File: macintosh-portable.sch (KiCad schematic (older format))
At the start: 0 parts

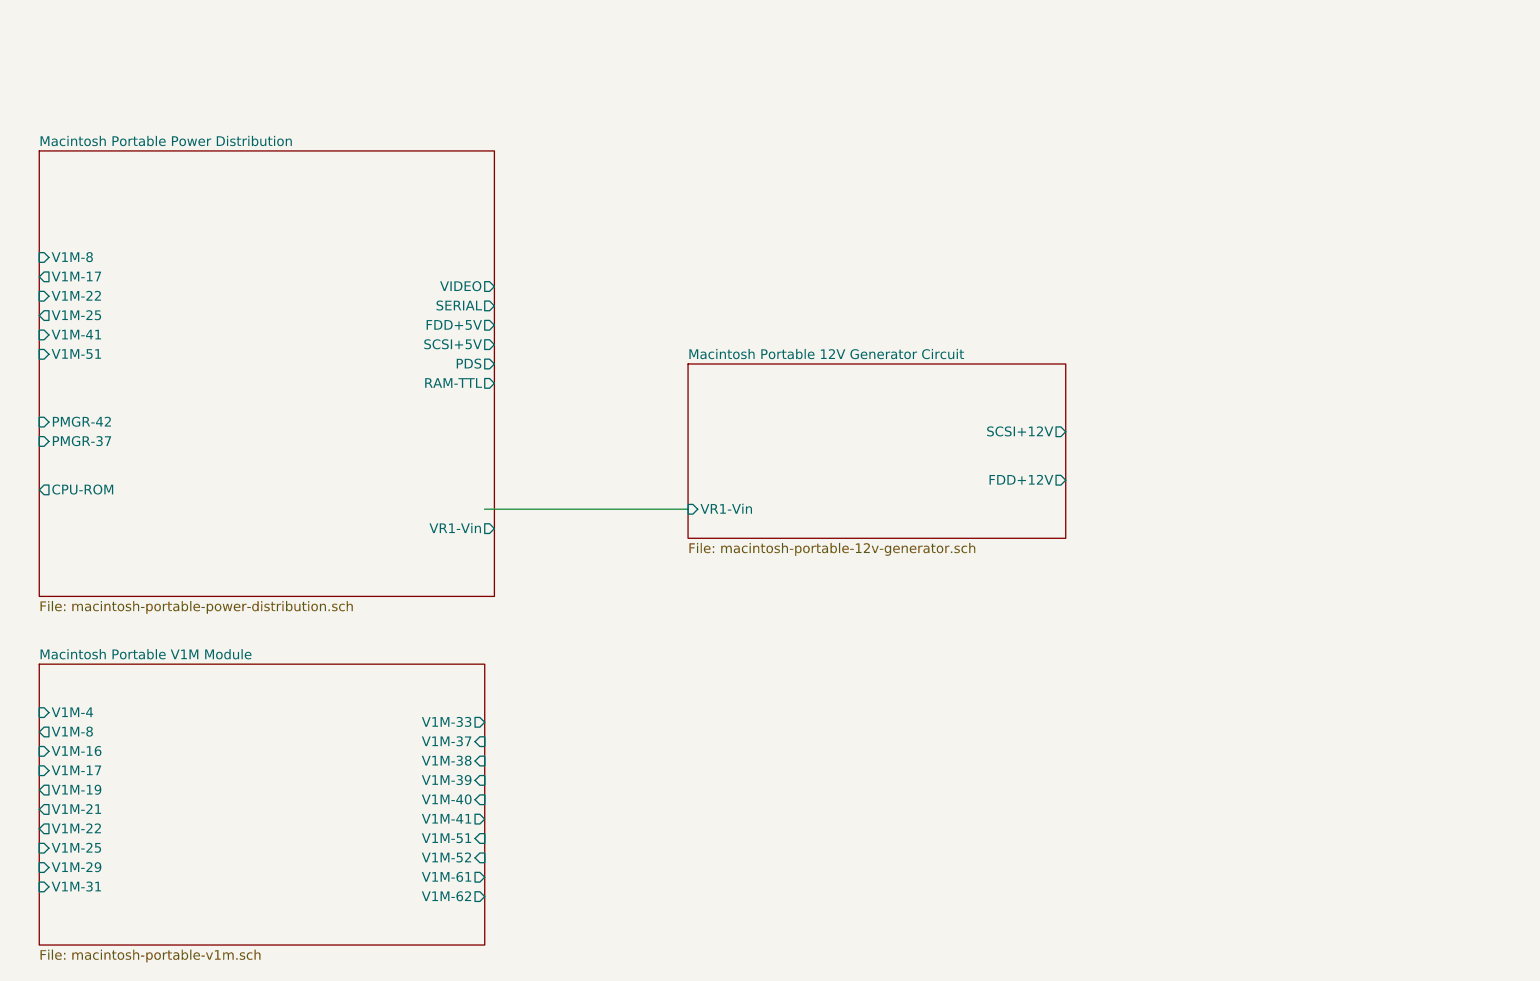
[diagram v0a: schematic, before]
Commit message: Finished V1M, more references on other sheets.
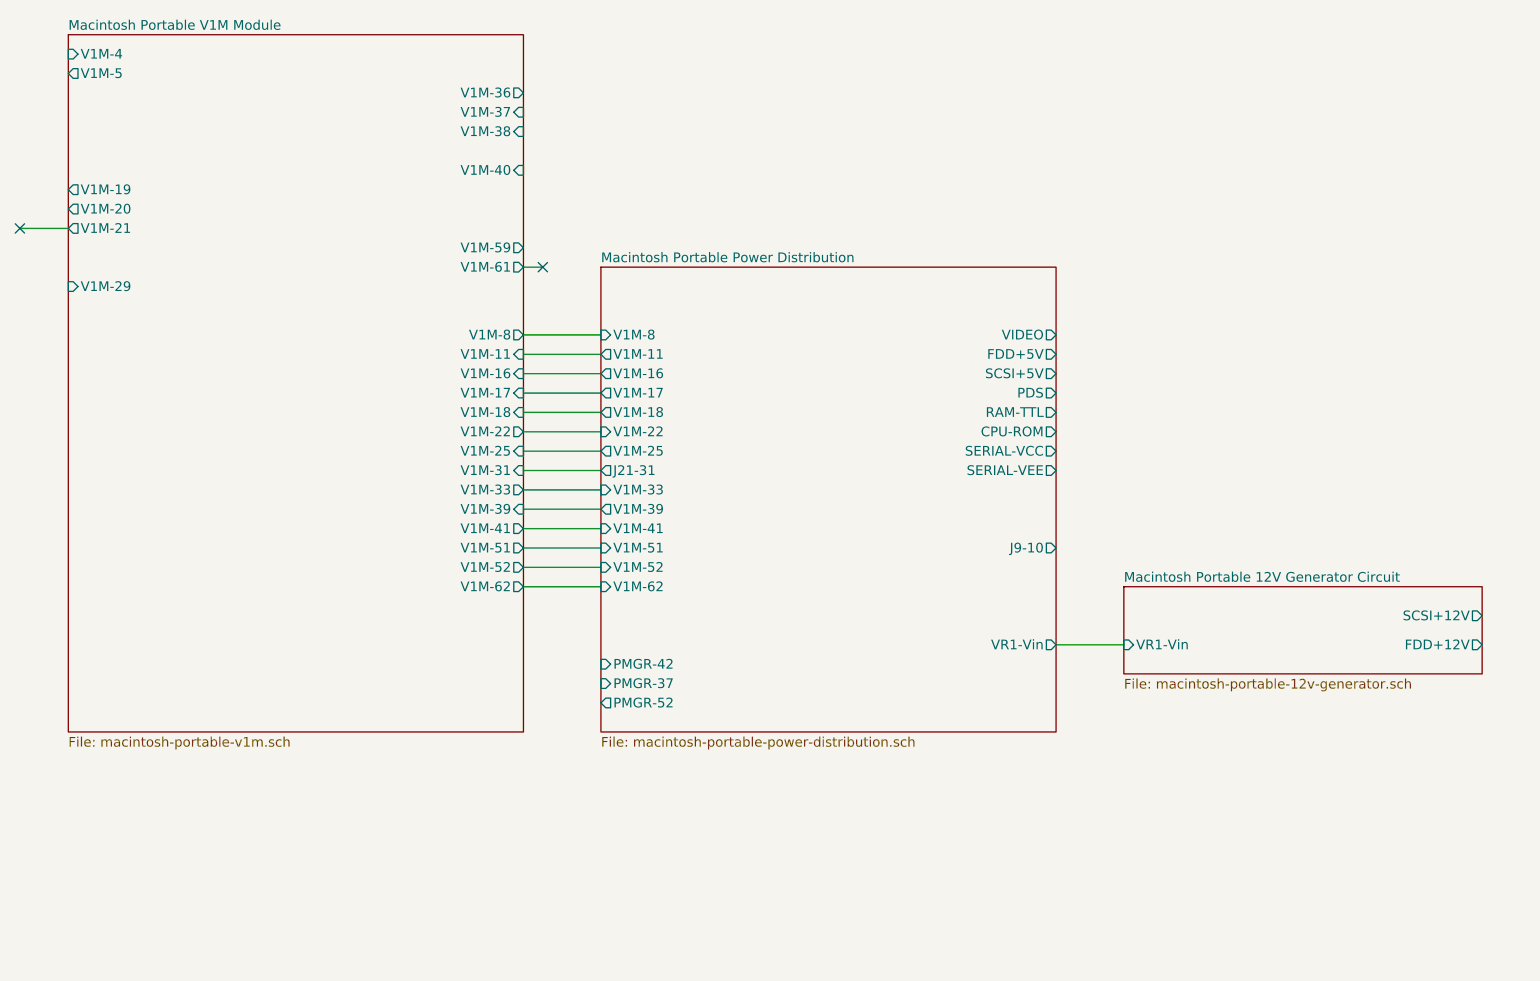
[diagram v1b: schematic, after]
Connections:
- wire segments 1 -> 17
- no-connect marks 0 -> 2
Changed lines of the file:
@@
 encoding utf-8
 Sheet 1 4
-Title ""
-Date ""
-Rev "0.1"
-Comp ""
-Comment1 ""
+Title "Macintosh Portable Power"
+Date "2019-05-27"
+Rev "0.12"
+Comp "https://oldcrap.org"
+Comment1 "Author: Pawel Pieczul"
 Comment2 ""
 Comment3 ""
@@
 $EndDescr
 $Sheet
-S 1200 1500 2350 2300
+S 4100 2100 2350 2400
 U 5CE45908
 F0 "Macintosh Portable Power Distribution" 50
 F1 "macintosh-portable-power-distribution.sch" 50
-F2 "VR1-Vin" O R 3550 3450 50
-F3 "V1M-41" I L 1200 2450 50
-F4 "V1M-51" I L 1200 2550 50
-F5 "PMGR-42" I L 1200 2900 50
-F6 "SCSI+5V" O R 3550 2500 50
-F7 "V1M-8" I L 1200 2050 50
-F8 "FDD+5V" O R 3550 2400 50
-F9 "CPU-ROM" O L 1200 3250 50
-F10 "PDS" O R 3550 2600 50
-F11 "VIDEO" O R 3550 2200 50
-F12 "SERIAL" O R 3550 2300 50
-F13 "V1M-25" O L 1200 2350 50
-F14 "V1M-17" O L 1200 2150 50
-F15 "V1M-22" I L 1200 2250 50
-F16 "RAM-TTL" O R 3550 2700 50
-F17 "PMGR-37" I L 1200 3000 50
+F2 "VR1-Vin" O R 6450 4050 50
+F3 "V1M-41" I L 4100 3450 50
+F4 "V1M-51" I L 4100 3550 50
+F5 "PMGR-42" I L 4100 4150 50
+F6 "SCSI+5V" O R 6450 2650 50
+F7 "V1M-8" I L 4100 2450 50
+F8 "FDD+5V" O R 6450 2550 50
+F9 "CPU-ROM" O R 6450 2950 50
+F10 "PDS" O R 6450 2750 50
+F11 "VIDEO" O R 6450 2450 50
+F12 "V1M-25" O L 4100 3050 50
+F13 "V1M-17" O L 4100 2750 50
+F14 "V1M-22" I L 4100 2950 50
+F15 "RAM-TTL" O R 6450 2850 50
+F16 "PMGR-37" I L 4100 4250 50
+F17 "SERIAL-VCC" O R 6450 3050 50
+F18 "V1M-52" I L 4100 3650 50
+F19 "V1M-39" O L 4100 3350 50
+F20 "V1M-16" O L 4100 2650 50
+F21 "V1M-62" I L 4100 3750 50
+F22 "J21-31" O L 4100 3150 50
+F23 "PMGR-52" O L 4100 4350 50
+F24 "V1M-33" I L 4100 3250 50
+F25 "J9-10" O R 6450 3550 50
+F26 "V1M-18" O L 4100 2850 50
+F27 "V1M-11" O L 4100 2550 50
+F28 "SERIAL-VEE" O R 6450 3150 50
 $EndSheet
 $Sheet
-S 4550 2600 1950 900
+S 6800 3750 1850 450
 U 5CFAA7F4
 F0 "Macintosh Portable 12V Generator Circuit" 50
 F1 "macintosh-portable-12v-generator.sch" 50
-F2 "VR1-Vin" I L 4550 3350 50
-F3 "SCSI+12V" O R 6500 2950 50
-F4 "FDD+12V" O R 6500 3200 50
+F2 "VR1-Vin" I L 6800 4050 50
+F3 "SCSI+12V" O R 8650 3900 50
+F4 "FDD+12V" O R 8650 4050 50
 $EndSheet
 Wire Wire Line
-	3500 3350 4550 3350
+	6450 4050 6800 4050
 $Sheet
-S 1200 4150 2300 1450
+S 1350 900  2350 3600
 U 5CE523FB
 F0 "Macintosh Portable V1M Module" 50
 F1 "macintosh-portable-v1m.sch" 50
-F2 "V1M-22" O L 1200 5000 50
-F3 "V1M-16" I L 1200 4600 50
-F4 "V1M-17" I L 1200 4700 50
-F5 "V1M-40" I R 3500 4850 50
-F6 "V1M-29" I L 1200 5200 50
-F7 "V1M-31" I L 1200 5300 50
-F8 "V1M-25" I L 1200 5100 50
-F9 "V1M-37" I R 3500 4550 50
-F10 "V1M-51" I R 3500 5050 50
-F11 "V1M-52" I R 3500 5150 50
-F12 "V1M-62" O R 3500 5350 50
-F13 "V1M-8" O L 1200 4500 50
-F14 "V1M-4" I L 1200 4400 50
-F15 "V1M-39" I R 3500 4750 50
-F16 "V1M-38" I R 3500 4650 50
-F17 "V1M-41" O R 3500 4950 50
-F18 "V1M-19" O L 1200 4800 50
-F19 "V1M-21" O L 1200 4900 50
-F20 "V1M-33" O R 3500 4450 50
-F21 "V1M-61" O R 3500 5250 50
+F2 "V1M-22" O R 3700 2950 50
+F3 "V1M-16" I R 3700 2650 50
+F4 "V1M-17" I R 3700 2750 50
+F5 "V1M-40" I R 3700 1600 50
+F6 "V1M-29" I L 1350 2200 50
+F7 "V1M-31" I R 3700 3150 50
+F8 "V1M-25" I R 3700 3050 50
+F9 "V1M-37" I R 3700 1300 50
+F10 "V1M-51" O R 3700 3550 50
+F11 "V1M-52" O R 3700 3650 50
+F12 "V1M-62" O R 3700 3750 50
+F13 "V1M-8" O R 3700 2450 50
+F14 "V1M-4" I L 1350 1000 50
+F15 "V1M-39" I R 3700 3350 50
+F16 "V1M-38" I R 3700 1400 50
+F17 "V1M-41" O R 3700 3450 50
+F18 "V1M-19" O L 1350 1700 50
+F19 "V1M-21" O L 1350 1900 50
+F20 "V1M-33" O R 3700 3250 50
+F21 "V1M-61" O R 3700 2100 50
+F22 "V1M-5" O L 1350 1100 50
+F23 "V1M-20" O L 1350 1800 50
+F24 "V1M-36" O R 3700 1200 50
+F25 "V1M-59" O R 3700 2000 50
+F26 "V1M-11" I R 3700 2550 50
+F27 "V1M-18" I R 3700 2850 50
 $EndSheet
+NoConn ~ 1100 1900
+NoConn ~ 3800 2100
+Wire Wire Line
+	3800 2100 3700 2100
+Wire Wire Line
+	1100 1900 1350 1900
+Wire Wire Line
+	3700 2450 4100 2450
+Wire Wire Line
+	3700 2550 4100 2550
+Wire Wire Line
+	4100 2650 3700 2650
+Wire Wire Line
+	4100 2750 3700 2750
+Wire Wire Line
+	4100 2850 3700 2850
+Wire Wire Line
+	3700 2950 4100 2950
+Wire Wire Line
+	4100 3050 3700 3050
+Wire Wire Line
+	4100 3150 3700 3150
+Wire Wire Line
+	3700 3250 4100 3250
+Wire Wire Line
+	4100 3350 3700 3350
+Wire Wire Line
+	3700 3450 4100 3450
+Wire Wire Line
+	3700 3550 4100 3550
+Wire Wire Line
+	3700 3650 4100 3650
+Wire Wire Line
+	3700 3750 4100 3750
 $EndSCHEMATC
